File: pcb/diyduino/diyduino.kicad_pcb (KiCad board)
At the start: 2 copper layers, 42 parts, among them J1 Conn_Coaxial_Power, U1 ATMEGA328-PU, U2 L7805, Y1 16MHz

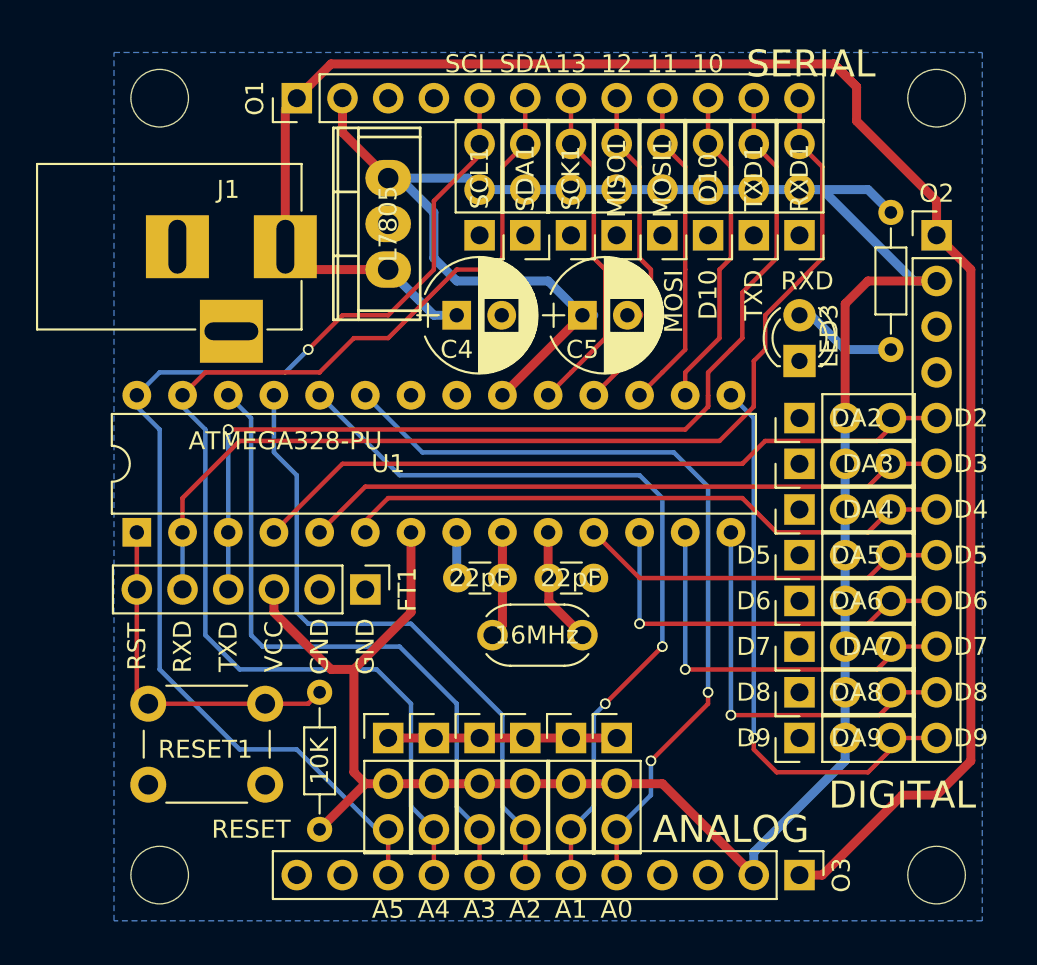
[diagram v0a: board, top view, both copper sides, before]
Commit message: Reworked the ditduino.
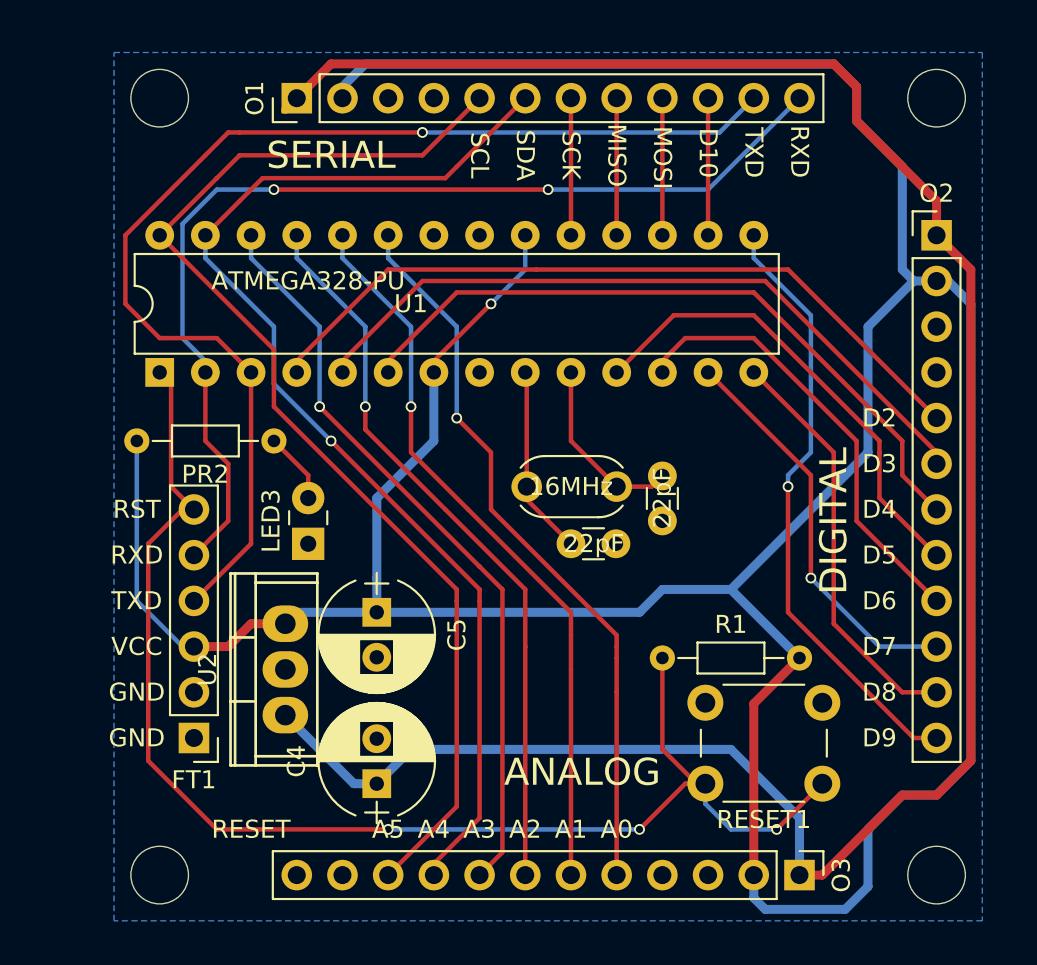
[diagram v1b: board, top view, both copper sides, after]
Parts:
- removed A0, A1, A2, A3, A4, A5, D10, DA2, DA3, DA4, DA5, DA6, DA7, DA8, DA9, MISO1, MOSI1, RXD1, SCK1, SCL1, SDA1, TXD1: DATA, Pin_Headers:Pin_Header_Straight_1x03_Pitch2.54mm
- removed J1: Conn_Coaxial_Power, Connectors:BARREL_JACK
- LED3: footprint LEDs:LED_D3.0mm -> LEDs:LED_Rectangular_W3.0mm_H2.0mm
- moved RESET1 37.7 mm to (148.6, 72.4), turned to 180 degrees
- moved PR2 34.7 mm to (118.1, 53.3), turned to 180 degrees
- moved LED3 29.1 mm to (120.0, 59.1)
- moved C4 26.4 mm to (123.8, 72.4), turned to 90 degrees
- moved U2 25.4 mm to (118.7, 66.0)
- moved C5 20.1 mm to (123.8, 62.9), turned to 270 degrees
- moved R1 19.1 mm to (139.7, 65.4), turned to 0 degrees
- moved FT1 12.6 mm to (113.7, 69.8), turned to 180 degrees
- moved U1 8.98 mm to (111.8, 49.5)
- moved Y1 8.47 mm to (137.2, 55.9)
- moved C3 4.96 mm to (139.7, 57.8), turned to 90 degrees
- moved C2 4.26 mm to (134.6, 59.1), turned to 0 degrees
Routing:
- net /RESET: track 19.6 -> 74.9 mm, vias 0 -> 3
- net /VCC: track 158.9 -> 198.9 mm, vias 0 -> 1
- net /VIN: track 107.4 -> 125.0 mm
- net Earth: track 15.4 -> 0.00 mm
- net /D13: track 19.2 -> 7.62 mm
- net /D12: track 18.6 -> 7.62 mm
- net /D11: track 18.1 -> 7.62 mm
- net /D10: track 18.1 -> 7.62 mm
- net /D1: track 56.0 -> 65.1 mm
- net /D5: track 20.6 -> 26.5 mm
- net /A2: track 35.8 -> 40.8 mm, vias 0 -> 1
- net /A3: track 36.9 -> 41.9 mm, vias 0 -> 1
- net Net-(C2-Pad1): track 5.94 -> 10.7 mm
- net /D3: track 35.9 -> 40.1 mm
- net /D4: track 34.6 -> 38.8 mm
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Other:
- board text added: "A0"
- board text added: "A1"
- board text added: "A2"
- board text added: "A3"
- board text added: "A4"
- board text added: "A5"
- board text added: "MISO"
- board text added: "SCK"
- board text removed: "10"
- board text removed: "11"
- board text removed: "12"
- board text removed: "13"
